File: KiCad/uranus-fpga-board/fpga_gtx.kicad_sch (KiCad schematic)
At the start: 1 part, among them U20 XC7K325T-3FFG900E

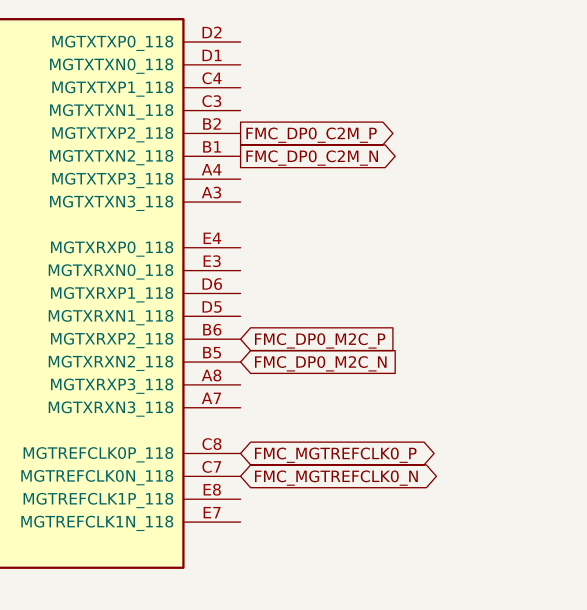
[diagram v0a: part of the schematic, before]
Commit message: Big things have mostly happened in schematic quality
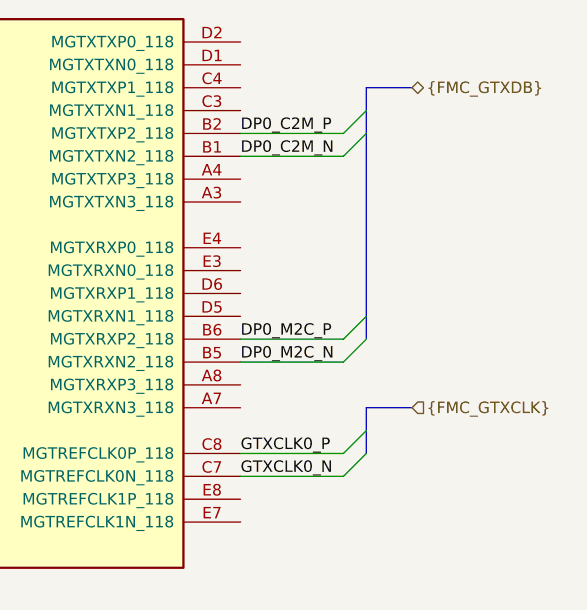
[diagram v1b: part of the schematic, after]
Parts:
- renumbered U20 to U12
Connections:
- net FMC_DP0_C2M_N renamed DP0_C2M_N
- net FMC_DP0_C2M_P renamed DP0_C2M_P
- net FMC_DP0_M2C_N renamed DP0_M2C_N
- net FMC_DP0_M2C_P renamed DP0_M2C_P
- net FMC_MGTREFCLK0_N renamed GTXCLK0_N
- net FMC_MGTREFCLK0_P renamed GTXCLK0_P

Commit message: I finally did it
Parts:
- U1: renamed from U12; footprint (none) -> Package_BGA:Xilinx_FFG900_FFG901
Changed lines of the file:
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@@
 		(dnp no)
 		(fields_autoplaced yes)
-		(property "Reference" "U12"
+		(property "Reference" "U1"
 			(at 104.14 88.9 0)
 			(hide yes)
@@
 			)
 		)
-		(property "Footprint" ""
+		(property "Footprint" "Package_BGA:Xilinx_FFG900_FFG901"
 			(at 104.14 90.17 0)
 			(hide yes)
@@
 			(project "uranus-fpga-board"
 				(path "/11d4e4d4-71ba-48aa-ae73-e6b6dc32b11b/ae4670d8-3f7e-4e25-83c4-e414aeb132b8/5601c772-9d70-4d6a-b42b-748160249e32"
-					(reference "U12")
+					(reference "U1")
 					(unit 12)
 				)
@@
 		(dnp no)
 		(fields_autoplaced yes)
-		(property "Reference" "U12"
+		(property "Reference" "U1"
 			(at 195.58 86.36 0)
 			(hide yes)
@@
 			)
 		)
-		(property "Footprint" ""
+		(property "Footprint" "Package_BGA:Xilinx_FFG900_FFG901"
 			(at 195.58 87.63 0)
 			(hide yes)
@@
 			(project "uranus-fpga-board"
 				(path "/11d4e4d4-71ba-48aa-ae73-e6b6dc32b11b/ae4670d8-3f7e-4e25-83c4-e414aeb132b8/5601c772-9d70-4d6a-b42b-748160249e32"
-					(reference "U12")
+					(reference "U1")
 					(unit 13)
 				)
